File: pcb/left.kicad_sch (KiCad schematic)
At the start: 0 parts

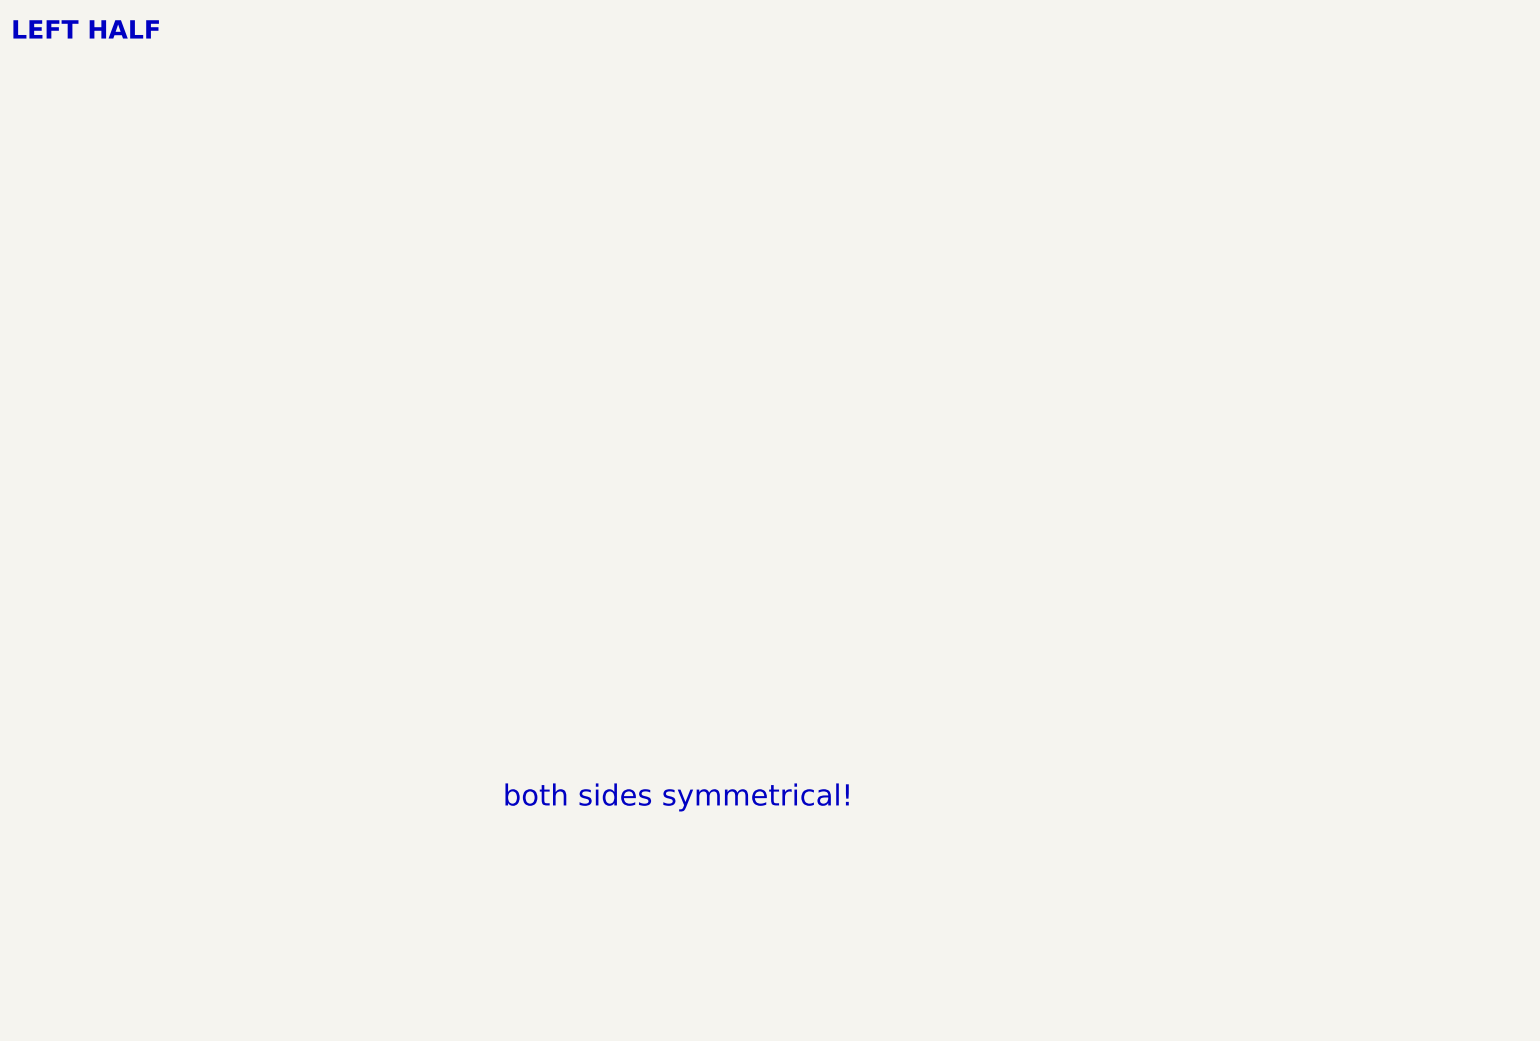
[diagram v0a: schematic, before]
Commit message: finished routing second half
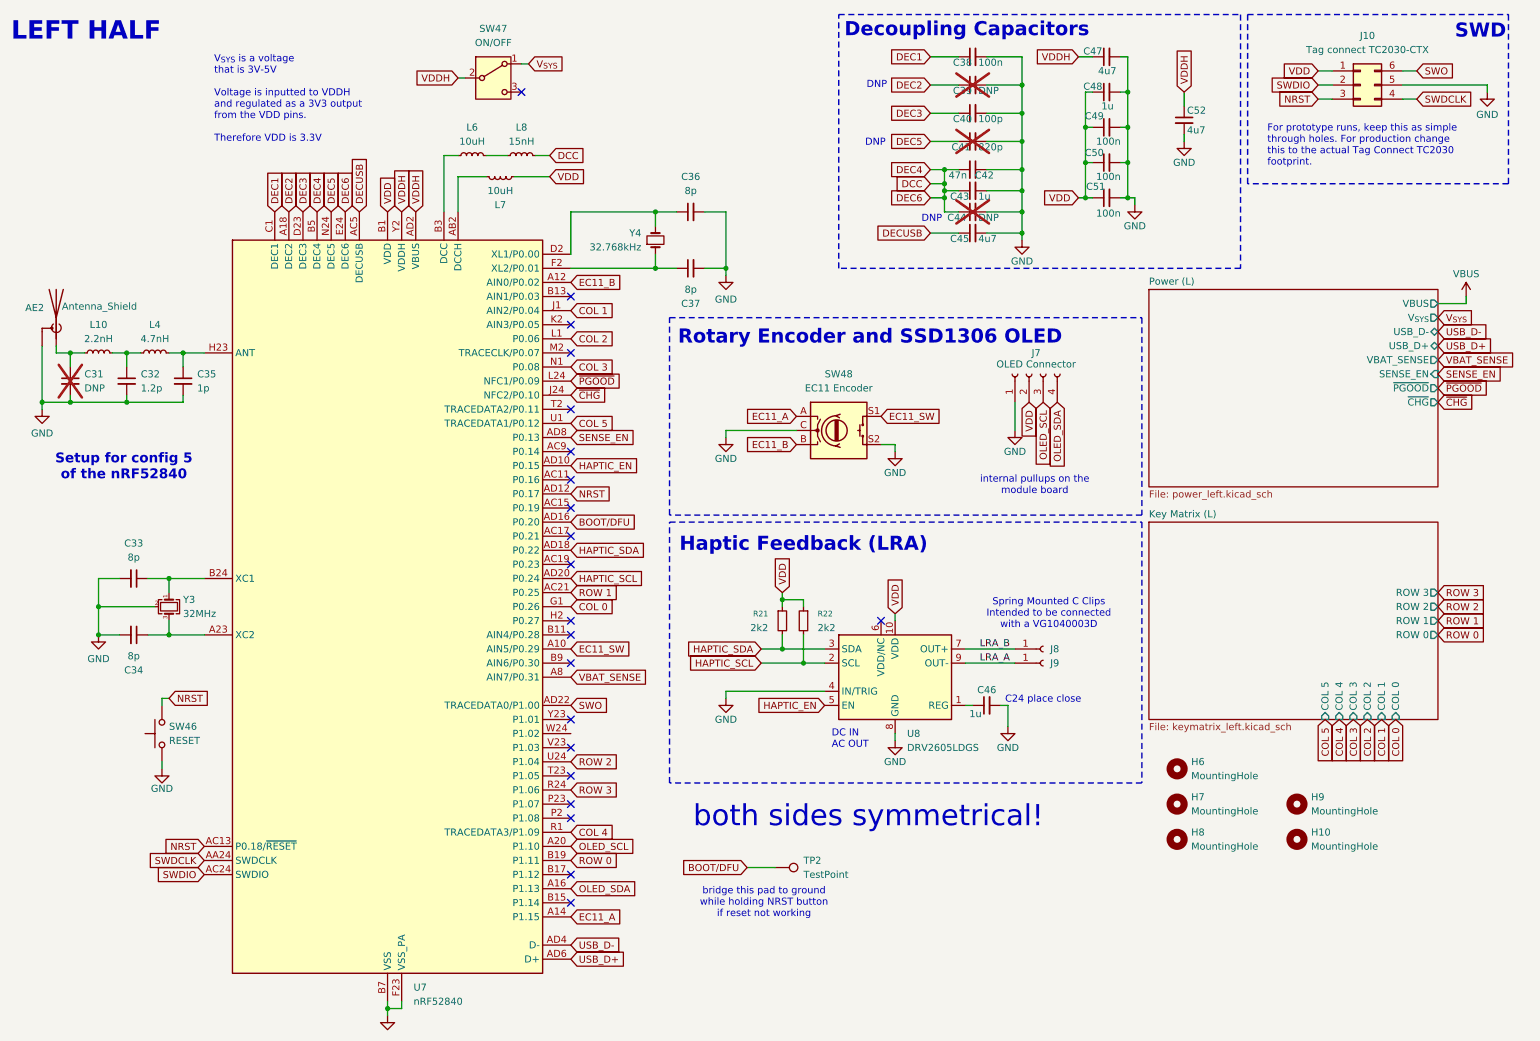
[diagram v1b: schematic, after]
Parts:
- added AE2: Antenna_Shield, kbd:BLE_ANTENNA, symbol Device:Antenna_Shield
- added C31, C39, C44: DNP, Capacitor_SMD:C_0402_1005Metric, symbol Device:C_Small
- added C32: 1.2p, Capacitor_SMD:C_0402_1005Metric, symbol Device:C_Small
- added C33, C34, C36, C37: 8p, Capacitor_SMD:C_0402_1005Metric, symbol Device:C_Small
- added C35: 1p, Capacitor_SMD:C_0402_1005Metric, symbol Device:C_Small
- added C38, C49, C50, C51: 100n, Capacitor_SMD:C_0402_1005Metric, symbol Device:C_Small
- added C40: 100p, Capacitor_SMD:C_0402_1005Metric, symbol Device:C_Small
- added C41: 820p, Capacitor_SMD:C_0402_1005Metric, symbol Device:C_Small
- added C42: 47n, Capacitor_SMD:C_0402_1005Metric, symbol Device:C_Small
- added C43, C46, C48: 1u, Capacitor_SMD:C_0603_1608Metric, symbol Device:C_Small
- added C45, C47, C52: 4u7, Capacitor_SMD:C_0805_2012Metric, symbol Device:C_Small
- added H10, H6, H7, H8, H9: MountingHole, MountingHole:MountingHole_2.2mm_M2, symbol Mechanical:MountingHole
- added J10: Tag connect TC2030-CTX, Connector_PinHeader_2.54mm:PinHeader_2x03_P2.54mm_Vertical, symbol Connector_Generic:Conn_02x03_Counter_Clockwise
- added J7: OLED Connector, kbd:OLED, symbol Connector:Conn_01x04_Socket
- added J8, J9: Conn_01x01_Socket, kbd:TE_2199248-6, symbol Connector:Conn_01x01_Socket
- added L10: 2.2nH, Inductor_SMD:L_0402_1005Metric, symbol Device:L_Small
- added L4: 4.7nH, Inductor_SMD:L_0402_1005Metric, symbol Device:L_Small
- added L6, L7: 10uH, Inductor_SMD:L_0603_1608Metric, symbol Device:L_Small
- added L8: 15nH, Inductor_SMD:L_0402_1005Metric, symbol Device:L_Small
- added R21, R22: 2k2, Resistor_SMD:R_0402_1005Metric, symbol Device:R_Small
- added SW46: RESET, Button_Switch_SMD:SW_Push_SPST_NO_Alps_SKRK, symbol Switch:SW_Push
- added SW47: ON/OFF, Button_Switch_SMD:SW_SPDT_CK_JS102011SAQN, symbol Switch:SW_SPDT
- added SW48: EC11 Encoder, Rotary_Encoder:RotaryEncoder_Alps_EC11E-Switch_Vertical_H20mm_MountingHoles, symbol Device:RotaryEncoder_Switch
- added TP2: TestPoint, TestPoint:TestPoint_Pad_2.0x2.0mm, symbol Connector:TestPoint
- added U7: nRF52840, Package_DFN_QFN:Nordic_AQFN-73-1EP_7x7mm_P0.5mm, symbol MCU_Nordic:nRF52840
- added U8: DRV2605LDGS, Package_SO:VSSOP-10_3x3mm_P0.5mm, symbol Driver_Haptic:DRV2605LDGS
- added Y3: 32MHz, Crystal:Crystal_SMD_3225-4Pin_3.2x2.5mm, symbol Device:Crystal_GND24_Small
- added Y4: 32.768kHz, Crystal:Crystal_SMD_3215-2Pin_3.2x1.5mm, symbol Device:Crystal_Small
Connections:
- new net: C35.1, L4.2, U7.H23 (ANT)
- new net: L6.1, U7.B3 (DCC)
- new net: L6.2, L8.1
- new net: C33.1, U7.B24 (XC1), Y3.1
- new net: C34.1, U7.A23 (XC2), Y3.3
- new net: C36.1, U7.D2 (XL1/P0.00), Y4.2
- new net: L7.1, U7.AB2 (DCCH)
- new net: C37.1, U7.F2 (XL2/P0.01), Y4.1
- new net: AE2.1 (A), C31.1, L10.1
- new net: C46.1, U8.1 (REG)
- new net: C32.1, L10.2, L4.1
- new net BOOT/DFU: TP2.1, U7.AD16 (P0.20)
- new net COL 0: U7.G1 (P0.26)
- new net COL 1: U7.J1 (AIN2/P0.04)
- new net COL 2: U7.L1 (P0.06)
- new net COL 3: U7.N1 (P0.08)
- new net COL 4: U7.R1 (TRACEDATA3/P1.09)
- new net COL 5: U7.U1 (TRACEDATA1/P0.12)
- new net DCC: C42.2, C43.1, C44.1, L8.2, U7.B5 (DEC4), U7.E24 (DEC6)
- new net DEC1: C38.1, U7.C1 (DEC1)
- new net DEC2: C39.1, U7.A18 (DEC2)
- new net DEC3: C40.1, U7.D23 (DEC3)
- new net DEC5: C41.1, U7.N24 (DEC5)
- new net DECUSB: C45.1, U7.AC5 (DECUSB)
- new net EC11_A: SW48.A, U7.A14 (P1.15)
- new net EC11_B: SW48.B, U7.A12 (AIN0/P0.02)
- new net EC11_SW: SW48.S1, U7.A10 (AIN5/P0.29)
- new net GND: AE2.2 (Shield), C31.2, C32.2, C33.2, C34.2, C35.2, C36.2, C37.2, C38.2, C39.2, C40.2, C41.2, C42.1, C43.2, C44.2, C45.2, C46.2, C47.2, C48.2, C49.2, C50.2, C51.2, C52.2, J10.5 (Pin_5), J7.1 (Pin_1), SW46.1, SW48.C, SW48.S2, U7.B7 (VSS), U7.EP (VSS), U7.F23 (VSS_PA), U8.4 (IN/TRIG), U8.8 (GND), Y3.2 (G), Y3.4 (G)
- new net HAPTIC_EN: U7.AD10 (P0.15), U8.5 (EN)
- new net HAPTIC_SCL: R22.2, U7.AD20 (P0.24), U8.2 (SCL)
- new net HAPTIC_SDA: R21.2, U7.AD18 (P0.22), U8.3 (SDA)
- new net LRA_A: J9.1 (Pin_1), U8.9 (OUT-)
- new net LRA_B: J8.1, U8.7 (OUT+)
- new net NRST: J10.3 (Pin_3), SW46.2, U7.AC13 (P0.18/~{RESET}), U7.AD12 (P0.17)
- new net OLED_SCL: J7.3 (Pin_3), U7.A20 (P1.10)
- new net OLED_SDA: J7.4 (Pin_4), U7.A16 (P1.13)
- new net ROW 0: U7.B19 (P1.11)
- new net ROW 1: U7.AC21 (P0.25)
- new net ROW 2: U7.U24 (P1.04)
- new net ROW 3: U7.R24 (P1.06)
- new net SENSE_EN: U7.AD8 (P0.13)
- new net SWDCLK: J10.4 (Pin_4), U7.AA24 (SWDCLK)
- new net SWDIO: J10.2 (Pin_2), U7.AC24 (SWDIO)
- new net SWO: J10.6 (Pin_6), U7.AD22 (TRACEDATA0/P1.00)
- new net USB_D+: U7.AD6 (D+)
- new net USB_D-: U7.AD4 (D-)
- new net VBAT_SENSE: U7.A8 (AIN7/P0.31)
- new net VDD: C48.1, C49.1, C50.1, C51.1, J10.1 (Pin_1), J7.2 (Pin_2), L7.2, R21.1, R22.1, U7.A22 (VDD), U7.AD14 (VDD), U7.AD23 (VDD), U7.B1 (VDD), U7.W1 (VDD), U8.10 (VDD)
- new net VDDH: C47.1, C52.1, SW47.2 (B), U7.AD2 (VBUS), U7.Y2 (VDDH)
- new net V_{SYS}: SW47.1 (A)
- new net ~{CHG}: U7.J24 (NFC2/P0.10)
- new net ~{PGOOD}: U7.L24 (NFC1/P0.09)
- no-connect marks 0 -> 21
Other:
- added sheet Key Matrix (L) (keymatrix_left.kicad_sch)
- added sheet Power (L) (power_left.kicad_sch)
- note added: "C24 place close"
- note added: "DC IN AC OUT"
- note added: "DNP"
- note added: "Decoupling Capacitors"
- note added: "For prototype runs, keep this as simple through holes. For production change this to the actual Tag Connect TC2030 footprint."
- note added: "Haptic Feedback (LRA)"
- note added: "Rotary Encoder and SSD1306 OLED"
- note added: "SWD"
- note added: "Setup for config 5 of the nRF52840"
- note added: "Spring Mounted C Clips Intended to be connected with a VG1040003D"
- note added: "V_{SYS} is a voltage that is 3V-5V Voltage is inputted to VDDH and regulated as a 3V3 output from the VDD pins. Therefore VDD is 3.3V"
- note added: "bridge this pad to ground while holding NRST button if reset not working"
- note added: "internal pullups on the module board"
